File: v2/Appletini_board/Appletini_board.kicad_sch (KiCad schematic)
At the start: 12 parts, among them J1 Conn_02x25_Counter_Clockwise, Q1 TP0610T, U1 Pico, U2 Teensy4.1

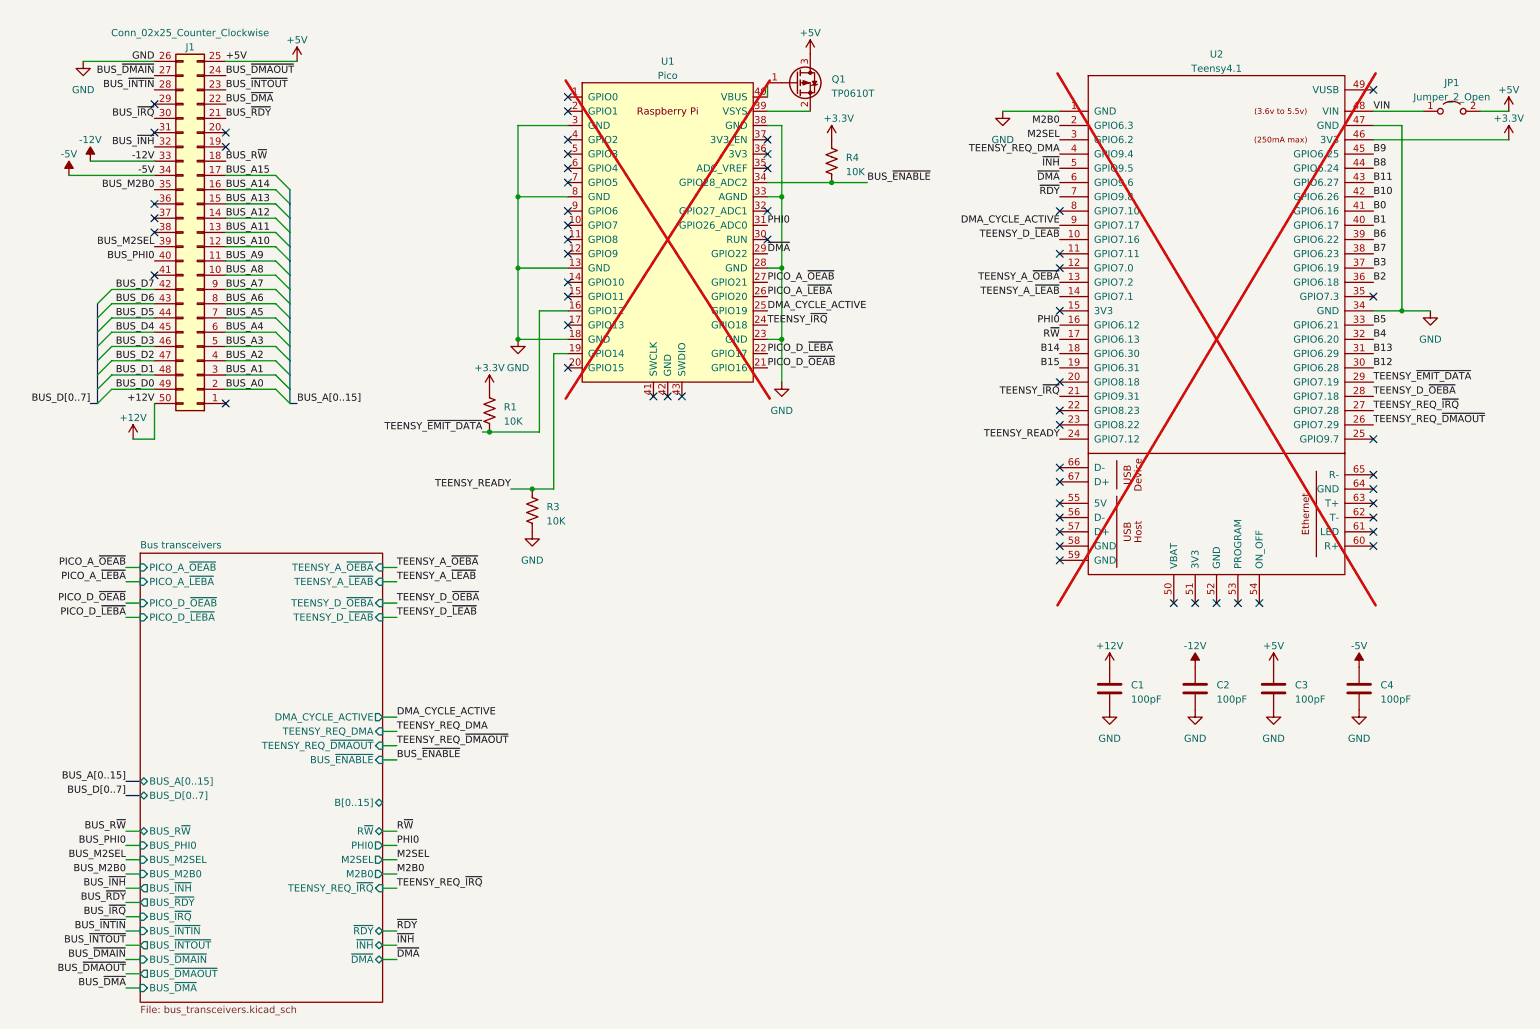
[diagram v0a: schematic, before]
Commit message: pcb debugging, first draft of PIO
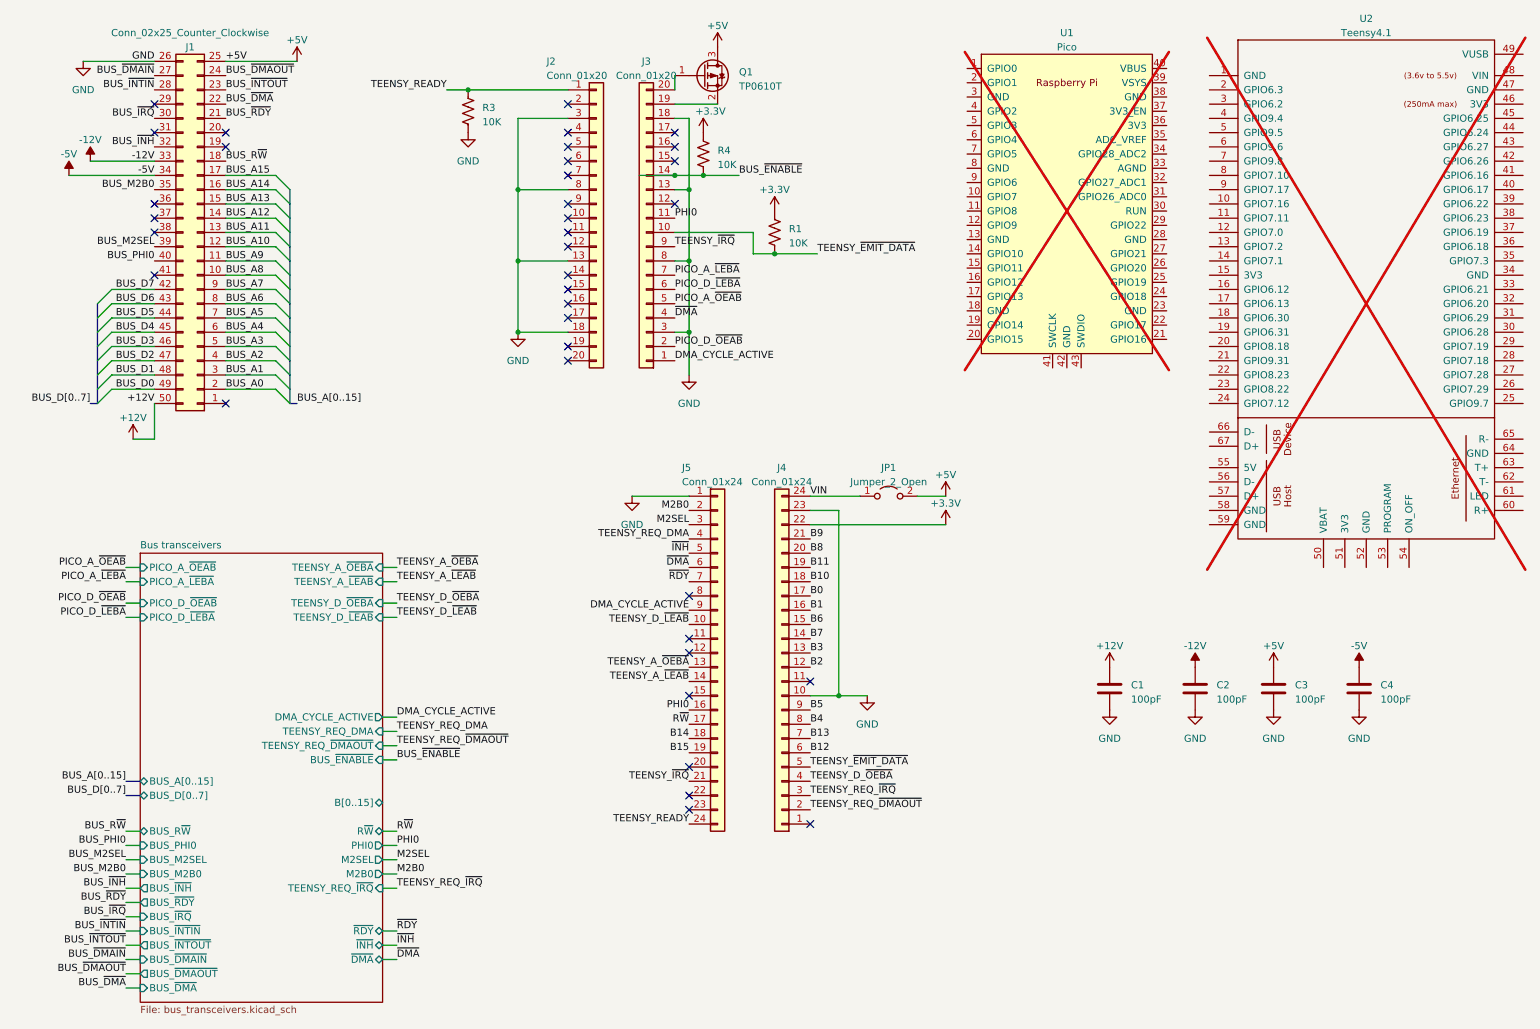
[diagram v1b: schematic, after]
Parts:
- added J2, J3: Conn_01x20, Connector_PinSocket_2.54mm:PinSocket_1x20_P2.54mm_Vertical, symbol Connector_Generic:Conn_01x20
- added J4, J5: Conn_01x24, Connector_PinSocket_2.54mm:PinSocket_1x24_P2.54mm_Vertical, symbol Connector_Generic:Conn_01x24
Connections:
- net +3.3V: now also J4.22 (Pin_22); no longer U2.46 (3V3)
- net B0: now also J4.17 (Pin_17); no longer U2.41 (GPIO6.16)
- net B1: now also J4.16 (Pin_16); no longer U2.40 (GPIO6.17)
- net B10: now also J4.18 (Pin_18); no longer U2.42 (GPIO6.26)
- net B11: now also J4.19 (Pin_19); no longer U2.43 (GPIO6.27)
- net B12: now also J4.6 (Pin_6); no longer U2.30 (GPIO6.28)
- net B13: now also J4.7 (Pin_7); no longer U2.31 (GPIO6.29)
- net B14: now also J5.18 (Pin_18); no longer U2.18 (GPIO6.30)
- net B15: now also J5.19 (Pin_19); no longer U2.19 (GPIO6.31)
- net B2: now also J4.12 (Pin_12); no longer U2.36 (GPIO6.18)
- net B3: now also J4.13 (Pin_13); no longer U2.37 (GPIO6.19)
- net B4: now also J4.8 (Pin_8); no longer U2.32 (GPIO6.20)
- net B5: now also J4.9 (Pin_9); no longer U2.33 (GPIO6.21)
- net B6: now also J4.15 (Pin_15); no longer U2.39 (GPIO6.22)
- net B7: now also J4.14 (Pin_14); no longer U2.38 (GPIO6.23)
- net B8: now also J4.20 (Pin_20); no longer U2.44 (GPIO6.24)
- net B9: now also J4.21 (Pin_21); no longer U2.45 (GPIO6.25)
- net BUS_~{ENABLE}: now also J3.14 (Pin_14); no longer U1.34 (GPIO28_ADC2)
- net DMA_CYCLE_ACTIVE: now also J3.1 (Pin_1), J5.9 (Pin_9); no longer U1.25 (GPIO19), U2.9 (GPIO7.17)
- net GND: now also J2.13 (Pin_13), J2.18 (Pin_18), J2.3 (Pin_3), J2.8 (Pin_8), J3.13 (Pin_13), J3.18 (Pin_18), J3.3 (Pin_3), J3.8 (Pin_8), J4.10 (Pin_10), J4.23 (Pin_23), J5.1 (Pin_1); no longer U1.13 (GND), U1.18 (GND), U1.23 (GND), U1.28 (GND), U1.3 (GND), U1.33 (AGND), U1.38 (GND), U1.8 (GND), U2.1 (GND), U2.34 (GND), U2.47 (GND)
- net M2B0: now also J5.2 (Pin_2); no longer U2.2 (GPIO6.3)
- net M2SEL: now also J5.3 (Pin_3); no longer U2.3 (GPIO6.2)
- net PHI0: now also J3.11 (Pin_11), J5.16 (Pin_16); no longer U1.31 (GPIO26_ADC0), U2.16 (GPIO6.12)
- net PICO_A_~{LEBA}: now also J3.7 (Pin_7); no longer U1.26 (GPIO20)
- net PICO_A_~{OEAB}: now also J3.5 (Pin_5); no longer U1.27 (GPIO21)
- net PICO_D_~{LEBA}: now also J3.6 (Pin_6); no longer U1.22 (GPIO17)
- net PICO_D_~{OEAB}: now also J3.2 (Pin_2); no longer U1.21 (GPIO16)
- net R~{W}: now also J5.17 (Pin_17); no longer U2.17 (GPIO6.13)
- net TEENSY_A_~{LEAB}: now also J5.14 (Pin_14); no longer U2.14 (GPIO7.1)
- net TEENSY_A_~{OEBA}: now also J5.13 (Pin_13); no longer U2.13 (GPIO7.2)
- net TEENSY_D_~{LEAB}: now also J5.10 (Pin_10); no longer U2.10 (GPIO7.16)
- net TEENSY_D_~{OEBA}: now also J4.4 (Pin_4); no longer U2.28 (GPIO7.18)
- net TEENSY_READY: now also J2.1 (Pin_1), J5.24 (Pin_24); no longer U1.19 (GPIO14), U2.24 (GPIO7.12)
- net TEENSY_REQ_DMA: now also J5.4 (Pin_4); no longer U2.4 (GPIO9.4)
- net TEENSY_REQ_~{DMAOUT}: now also J4.2 (Pin_2); no longer U2.26 (GPIO7.29)
- net TEENSY_REQ_~{IRQ}: now also J4.3 (Pin_3); no longer U2.27 (GPIO7.28)
- net TEENSY_~{EMIT_DATA}: now also J3.10 (Pin_10), J4.5 (Pin_5); no longer U1.16 (GPIO12), U2.29 (GPIO7.19)
- net TEENSY_~{IRQ}: now also J3.9 (Pin_9), J5.21 (Pin_21); no longer U1.24 (GPIO18), U2.21 (GPIO9.31)
- net VIN: now also J4.24 (Pin_24); no longer U2.48 (VIN)
- net ~{DMA}: now also J3.4 (Pin_4), J5.6 (Pin_6); no longer U1.29 (GPIO22), U2.6 (GPIO9.6)
- net ~{INH}: now also J5.5 (Pin_5); no longer U2.5 (GPIO9.5)
- net ~{RDY}: now also J5.7 (Pin_7); no longer U2.7 (GPIO9.8)
- net at Q1.2 (S): now also J3.19 (Pin_19); no longer U1.39 (VSYS)
- net at Q1.1 (G): now also J3.20 (Pin_20); no longer U1.40 (VBUS)
- no-connect marks 59 -> 37
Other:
- moved on the sheet: JP1, Q1, R4
